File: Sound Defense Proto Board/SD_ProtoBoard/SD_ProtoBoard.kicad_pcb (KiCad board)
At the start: 2 copper layers, 15.2 x 33.2 mm, 21 parts, among them IC1 ATTINY402-SSNR, IC2 PAM8906M1018-13, IC3 MCP73831T-2ACI_OT, J1 Conn_01x03_Pin, J3 USB_C_Receptacle_PowerOnly_6P, J4 S2B-PH-SM4-TB_LF__SN_, X1 CPT-1404-85T

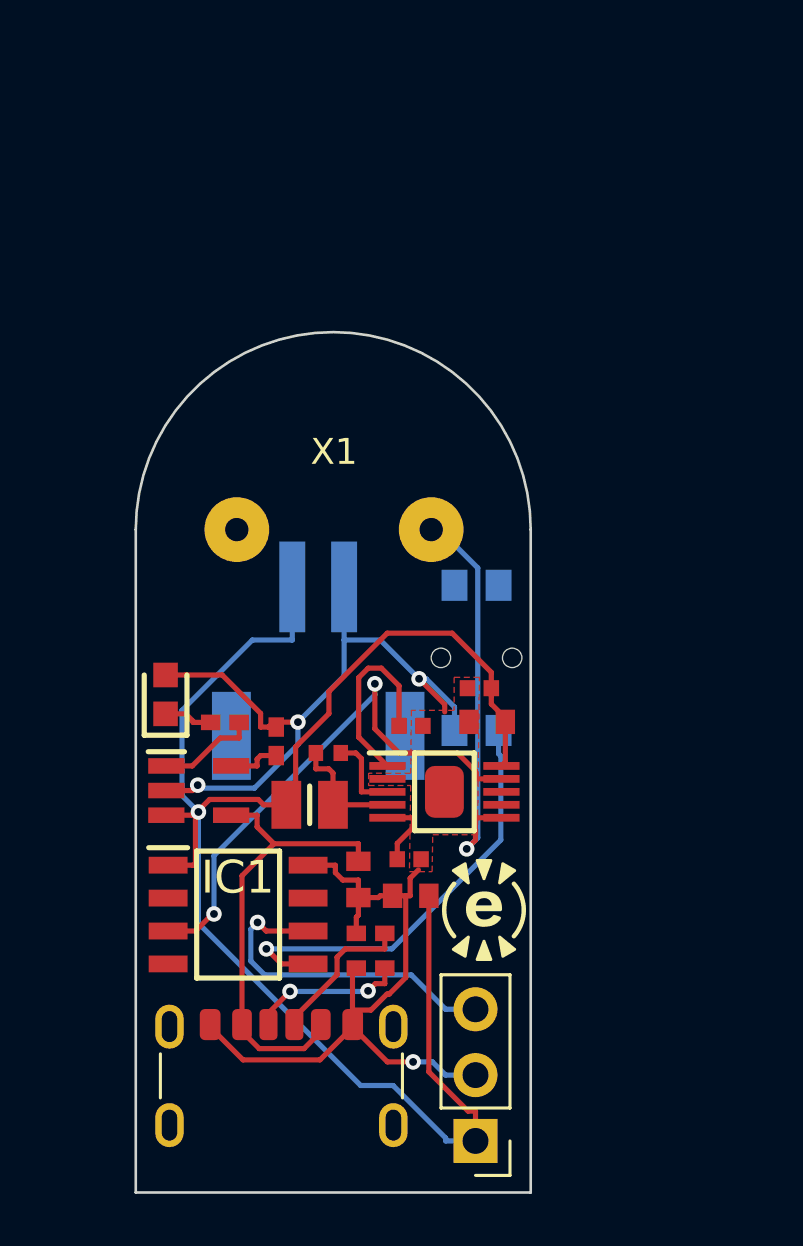
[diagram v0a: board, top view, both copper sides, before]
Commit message: Production Board v1-0
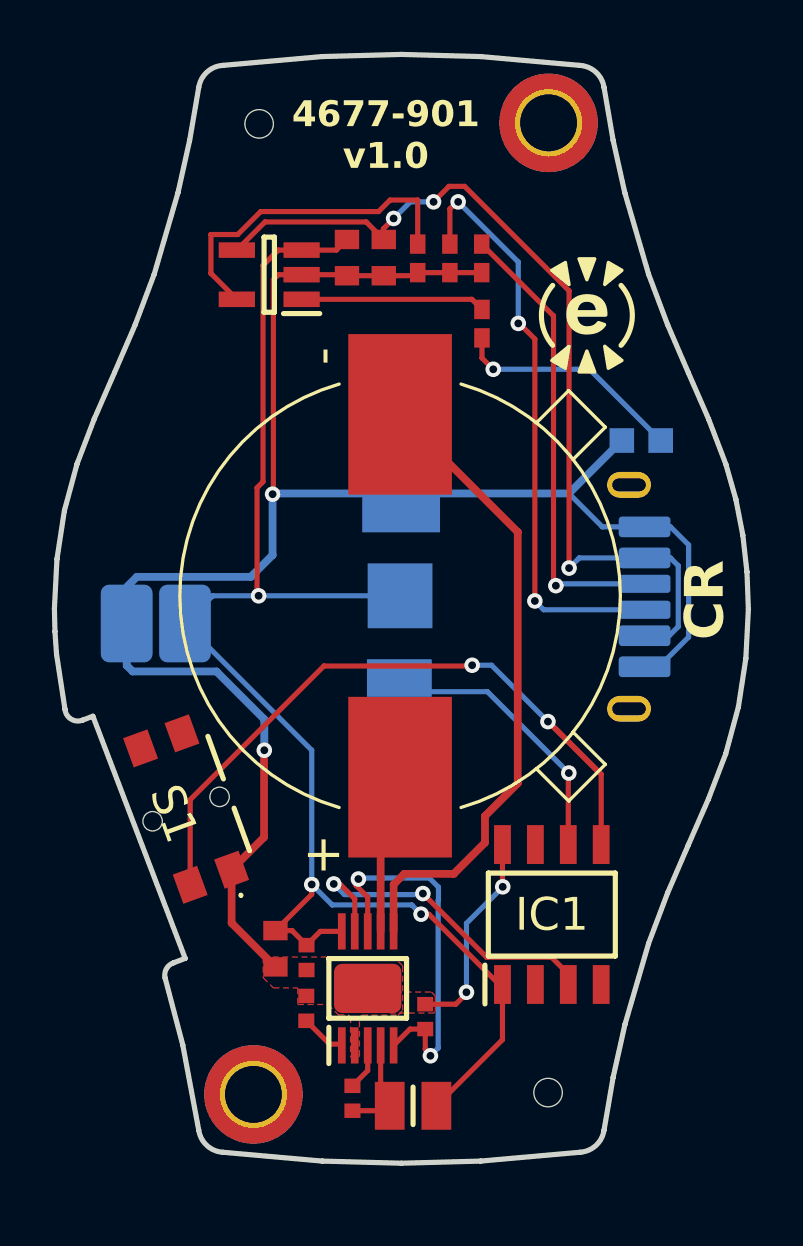
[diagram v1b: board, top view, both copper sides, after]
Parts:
- removed J3: USB_C_Receptacle_PowerOnly_6P, Connector_USB:USB_C_Receptacle_GCT_USB4125-xx-x-0190_6P_TopMnt_Horizontal
- removed J4: S2B-PH-SM4-TB_LF__SN_, SD-JST3:S2BPHSM4TBLFSN
- removed X1: CPT-1404-85T, SD-PIEZO:SD-CPT-1404-85T
- added H1: MountingHole, MountingHole:MountingHole_2.2mm_M2_DIN965_Pad_TopBottom, F.Cu at (147.9, 77.7)
- added H3: MountingHole, MountingHole:MountingHole_2.2mm_M2_DIN965_Pad_TopBottom, F.Cu at (136.5, 115.1)
- added LS1: CPT-1762-90-SMT-TR, SD-SMD-BUZZER:XDCR_CPT-1762-90-SMT-TR, F.Cu at (142.2, 95.9)
- added TP1: UPDI, TestPoint:TestPoint_Pad_2.5x2.5mm, B.Cu at (142.1, 99.6)
- added TP2: VCC, TestPoint:TestPoint_Pad_2.5x2.5mm, B.Cu at (142.2, 95.9)
- added TP3: GND, TestPoint:TestPoint_Pad_3.0x3.0mm, B.Cu at (142.2, 92.0)
- added U1: LP401230, Battery:LP402025, B.Cu at (138.7, 93.4)
- C1: value 0.1uF 0402B104K160CT -> 0.1uF
- C2, C4, C5: value 1uF GRM155R61E105KA12D -> 1uF; footprint SD-CAP1:CAPC1005X55N -> SD-01-CAP:CAPC1005X55N
- C3, C6, C7: value 10uF GRM188R61E106MA73D -> 10uF
- J1: value Conn_01x03_Pin -> MC-306LS-H50; footprint Connector_PinHeader_2.54mm:PinHeader_1x03_P2.54mm_Vertical -> SD-USB-C-SHORT:MC-306LS-H50; moved to B.Cu
- L1: footprint SD-IND:INDC2016X95N -> SD-INDUCTOR:INDC2016X95N
- LED1: value 150060VS75000 -> CHARGE INDICATOR; moved to B.Cu
- R1, R3: value 5.1KOhm -> 5.1K
- R4: value 10K Ohm -> 10K
- S1: value 436331045822 -> SIDE SWITCH; moved to F.Cu
- moved R1 27.7 mm to (145.3, 82.9), turned to 90 degrees
- moved R3 26.2 mm to (144.1, 82.9), turned to 90 degrees
- moved C7 24.7 mm to (140.1, 82.9), turned to -90 degrees
- moved C6 24.0 mm to (141.5, 82.9)
- moved J1 21.8 mm to (151.0, 95.9), turned to 90 degrees
- moved LED1 20.8 mm to (151.5, 89.9), turned to 180 degrees
- moved IC3 20.1 mm to (137.1, 83.5), turned to 180 degrees
- moved R4 19.4 mm to (142.9, 82.9), turned to -90 degrees
- moved R2 18.3 mm to (145.3, 85.4), turned to 90 degrees
- moved S1 13.6 mm to (133.4, 104.3), turned to -70 degrees
- moved C1 13.4 mm to (140.3, 115.3), turned to 90 degrees
- moved C4 12.4 mm to (138.6, 109.9), turned to -90 degrees
- moved L1 12.3 mm to (142.7, 115.6), turned to 180 degrees
- moved IC1 12.1 mm to (148.0, 108.2), turned to 90 degrees
- moved C3 12.0 mm to (137.4, 109.5), turned to -90 degrees
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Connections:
- net Net-(IC1-PA2) renamed /BUTTON
- net Net-(IC1-PA7) renamed /PWM
- R1 pad 2: Net-(J3-CC1) -> Net-(J1-CC2)
- R3 pad 2: Net-(J3-CC2) -> Net-(J1-CC1)
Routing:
- net GND: track 55.1 -> 78.6 mm
- net Net-(J1-CC1): track 0.00 -> 23.2 mm, vias 0 -> 3
- net Net-(J1-CC2): track 0.00 -> 17.9 mm, vias 0 -> 1
- net Net-(IC3-VDD): track 17.9 -> 35.6 mm, vias 0 -> 3
- net Net-(IC2-FB): track 2.86 -> 15.0 mm, vias 0 -> 2
- net /BUTTON: track 16.9 -> 28.6 mm, vias 1 -> 2
- net Net-(IC3-PROG): track 2.06 -> 13.1 mm
- net Net-(IC2-OUTN): track 15.8 -> 24.9 mm, vias 1 -> 0
- net /VBAT: track 65.3 -> 57.4 mm, vias 1 -> 3
- net /PWM: track 21.1 -> 13.3 mm
- net Net-(LED1-K): track 1.90 -> 8.99 mm, vias 0 -> 1
- net Net-(IC2-OUTP): track 0.00 -> 6.26 mm
- net Net-(J3-CC1): track 6.01 -> 0.00 mm, vias 2 -> 0
- net Net-(J3-CC2): track 5.86 -> 0.00 mm
- net Net-(IC2-VCC): track 7.40 -> 1.76 mm
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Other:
- board size 15.2 x 33.2 mm -> 26.8 x 42.8 mm
- board text added: "+"
- board text added: "-"
- board text added: "-WIRE ROUTE-"
- board text added: "4677-901 v1.0"
- board text added: "BAT"
- board text added: "BAT TOP"
- board text added: "CR"
- board text added: "CREATIVE ENGINEERING LLC"
- board text added: "PROPRIETARY PROTOTYPE"
- board text added: "VCC"
- board text removed: "2024-12-14"
- board text removed: "3.7v"
- board text removed: "PIN ASSIGNMENTS PAM-DIN -> PA7 (1) BUTTON -> PA2 (3)"
- board text removed: "Sound Defense Dev Board v3.0"
